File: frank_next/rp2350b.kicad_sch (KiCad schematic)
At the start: 38 parts, among them J1 Debug, J2 UART, U1 W25Q128JVPIQ, U2 ESP-PSRAM64H, U3 RP2350B, Y1 ASE-12MHz

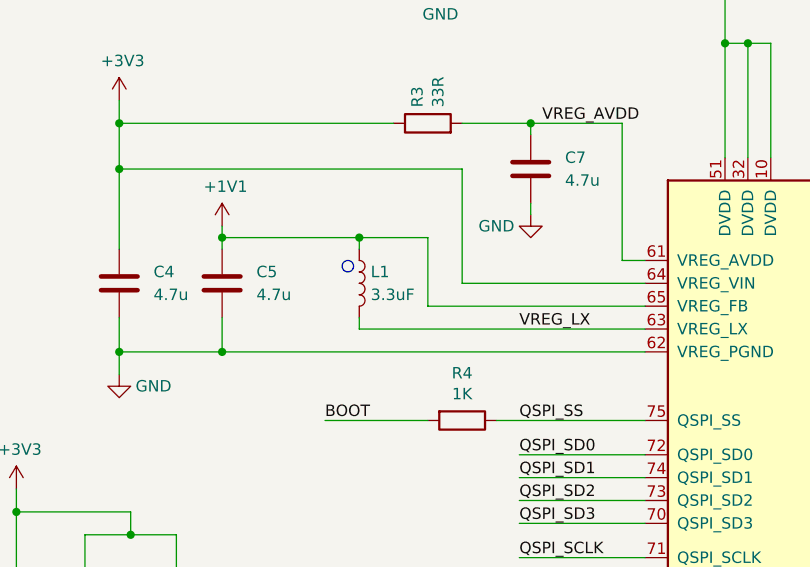
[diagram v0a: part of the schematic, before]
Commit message: Board updates
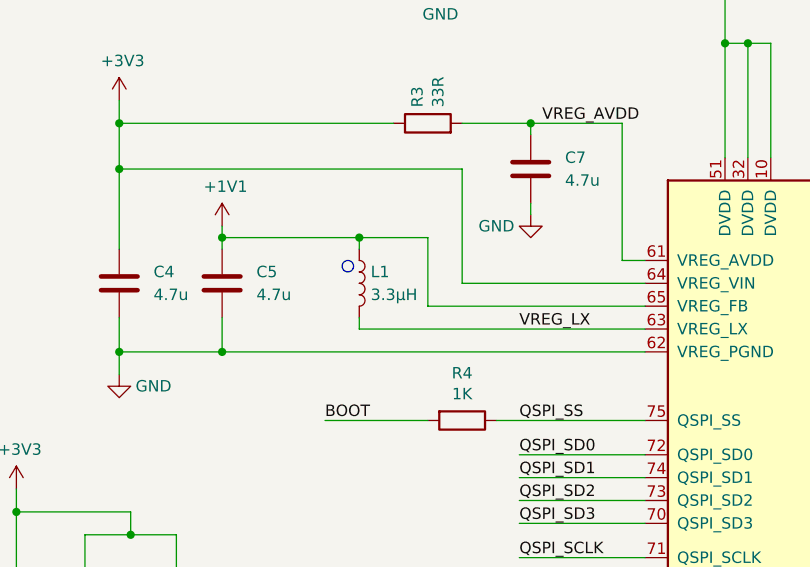
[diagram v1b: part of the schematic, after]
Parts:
- L1: value 3.3uF -> 3.3µH
- U1: footprint FRANK:SON127P600X500X80-9N-D -> FRANK:WSON-8-1EP_6x5mm_P1.27mm_EP3.45x4.35mm
- Y1: footprint FRANK:Oscillator_SMD_3225_4Pin -> FRANK:Oscillator_SMD_3225-4Pin_3.2x2.5mm
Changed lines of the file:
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@@
 		(fields_autoplaced yes)
 		(property "Reference" "L1"
-			(at 147.32 96.52 0)
+			(at 147.32 96.5199 0)
 			(show_name no)
 			(do_not_autoplace no)
@@
 			)
 		)
-		(property "Value" "3.3uF"
-			(at 147.32 99.06 0)
+		(property "Value" "3.3µH"
+			(at 147.32 99.0599 0)
 			(show_name no)
 			(do_not_autoplace no)
@@
 			)
 		)
-		(property "Footprint" "FRANK:SON127P600X500X80-9N-D"
+		(property "Footprint" "FRANK:WSON-8-1EP_6x5mm_P1.27mm_EP3.45x4.35mm"
 			(at 147.32 277.8 0)
 			(hide yes)
@@
 			)
 		)
-		(property "Footprint" "FRANK:Oscillator_SMD_3225_4Pin"
+		(property "Footprint" "FRANK:Oscillator_SMD_3225-4Pin_3.2x2.5mm"
 			(at 143.51 146.05 0)
 			(hide yes)
